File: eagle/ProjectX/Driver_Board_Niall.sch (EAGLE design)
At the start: 201 parts, among them IC2 NCV78M05BDTRKG, J1 694102303002, U1 TC4427AEOA, U10 TC4427AEOA, U11 TC4427AEOA, U12 TC4427AEOA, U1200 CD74HC4067SM96, U13 TC4427AEOA, U14 TC4427AEOA, U15 TC4427AEOA, U16 TC4427AEOA, U17 TC4427AEOA, U18 TC4427AEOA, U19 TC4427AEOA, U2 TC4427AEOA, U20 TC4427AEOA, U200 ADA4091-2ARZ-RL, U21 TC4427AEOA, U22 TC4427AEOA, U23 TC4427AEOA, U24 TC4427AEOA, U25 TC4427AEOA, U26 TC4427AEOA, U27 TC4427AEOA, U28 TC4427AEOA, U29 TC4427AEOA, U3 TC4427AEOA, U30 TC4427AEOA, U31 TC4427AEOA, U32 TC4427AEOA, U33 TC4427AEOA, U34 TC4427AEOA, U35 TC4427AEOA, U36 TC4427AEOA, U37 TC4427AEOA, U38 TC4427AEOA, U39 TC4427AEOA, U4 TC4427AEOA, U40 TC4427AEOA, U41 TC4427AEOA, U42 TC4427AEOA, U43 TC4427AEOA, U44 TC4427AEOA, U45 TC4427AEOA, U46 TC4427AEOA, U47 TC4427AEOA, U48 TC4427AEOA, U49 TC4427AEOA, U5 TC4427AEOA, U50 TC4427AEOA, U6 TC4427AEOA, U7 TC4427AEOA, U8 TC4427AEOA, U9 TC4427AEOA

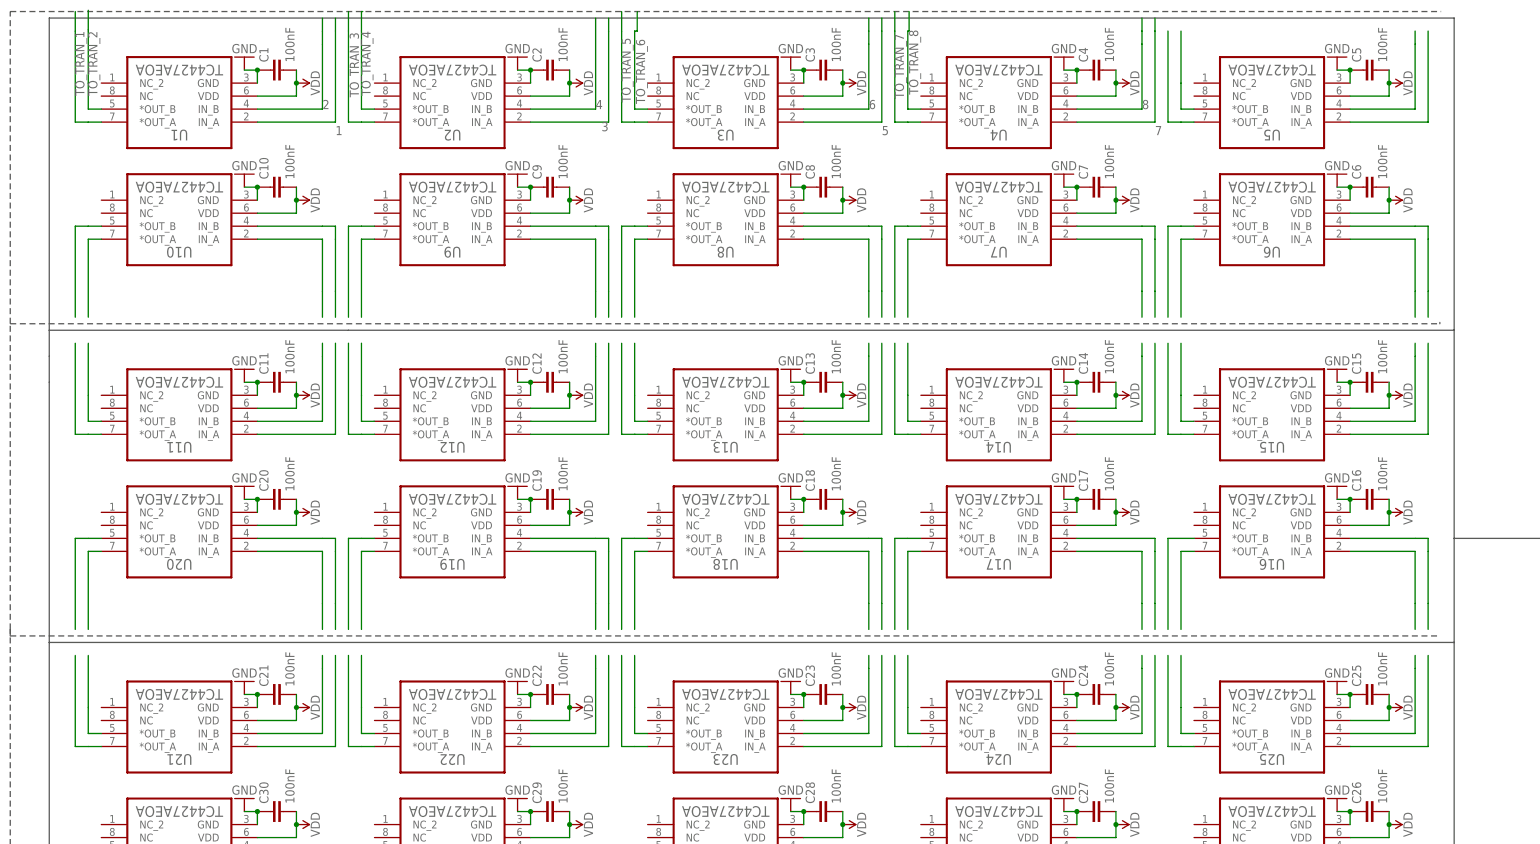
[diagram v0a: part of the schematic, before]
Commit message: Niall board edits
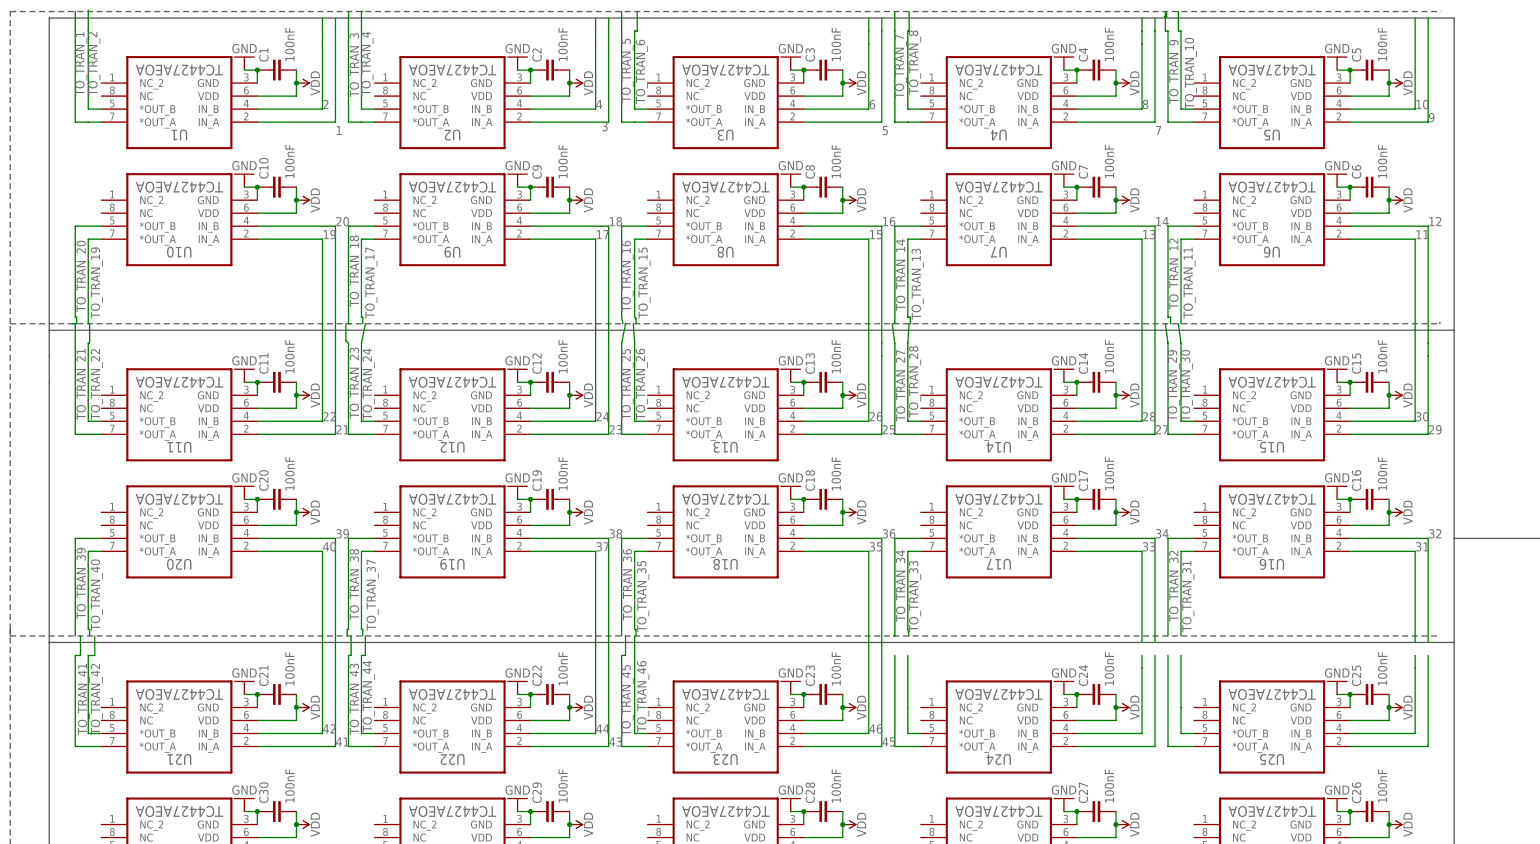
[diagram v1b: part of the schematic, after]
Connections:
- net 101 renamed 15
- net 102 renamed 16
- net 103 renamed 17
- net 104 renamed 18
- net 105 renamed 19
- net 106 renamed 20
- net 107 renamed 21
- net 108 renamed 22
- net 109 renamed 23
- net 110 renamed 24
- net 111 renamed 25
- net 112 renamed 26
- net 113 renamed 27
- net 114 renamed 28
- net 115 renamed 29
- net 116 renamed 30
- net 117 renamed 31
- net 118 renamed 32
- net 119 renamed 33
- net 120 renamed 34
- net 121 renamed 35
- net 122 renamed 36
- net 123 renamed 37
- net 124 renamed 38
- net 125 renamed 40
- net 126 renamed 39
- net 127 renamed 41
- net 128 renamed 42
- net 129 renamed 43
- net 130 renamed 44
- net 131 renamed 45
- net 132 renamed 46
- net DRIVE_10 renamed TO_TRAN_20
- net DRIVE_11 renamed TO_TRAN_22
- net DRIVE_12 renamed TO_TRAN_24
- net DRIVE_13 renamed TO_TRAN_26
- net DRIVE_14 renamed TO_TRAN_28
- net DRIVE_15 renamed TO_TRAN_30
- net DRIVE_16 renamed TO_TRAN_32
- net DRIVE_17 renamed TO_TRAN_34
- net DRIVE_18 renamed TO_TRAN_36
- net DRIVE_19 renamed TO_TRAN_38
- net DRIVE_20 renamed TO_TRAN_39
- net DRIVE_21 renamed TO_TRAN_42
- net DRIVE_22 renamed TO_TRAN_44
- net DRIVE_23 renamed TO_TRAN_46
- net DRIVE_5 renamed TO_TRAN_10
- net DRIVE_6 renamed TO_TRAN_12
- net DRIVE_7 renamed TO_TRAN_14
- net DRIVE_8 renamed TO_TRAN_16
- net DRIVE_9 renamed TO_TRAN_18
- net N$13 renamed TO_TRAN_11
- net N$15 renamed TO_TRAN_13
- net N$16 renamed TO_TRAN_15
- net N$17 renamed TO_TRAN_17
- net N$18 renamed TO_TRAN_19
- net N$19 renamed TO_TRAN_21
- net N$20 renamed TO_TRAN_23
- net N$21 renamed TO_TRAN_25
- net N$22 renamed TO_TRAN_27
- net N$23 renamed TO_TRAN_29
- net N$24 renamed TO_TRAN_31
- net N$25 renamed TO_TRAN_33
- net N$26 renamed TO_TRAN_35
- net N$27 renamed TO_TRAN_37
- net N$28 renamed TO_TRAN_40
- net N$29 renamed TO_TRAN_41
- net N$39 renamed TO_TRAN_43
- net N$40 renamed TO_TRAN_45
- net N$9 renamed TO_TRAN_9
- new net 10: U5.IN_B
- new net 11: U6.IN_A
- new net 12: U6.IN_B
- new net 13: U7.IN_A
- new net 14: U7.IN_B
- new net 9: U5.IN_A
- net 100: no longer U7.IN_B
- net 95: no longer U5.IN_A
- net 96: no longer U5.IN_B
- net 97: no longer U6.IN_A
- net 98: no longer U6.IN_B
- net 99: no longer U7.IN_A
